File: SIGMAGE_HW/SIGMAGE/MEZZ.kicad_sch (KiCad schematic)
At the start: 4 parts, among them J12 61306421821, J13 61306421121, J14 61306421821, J8 61306421121

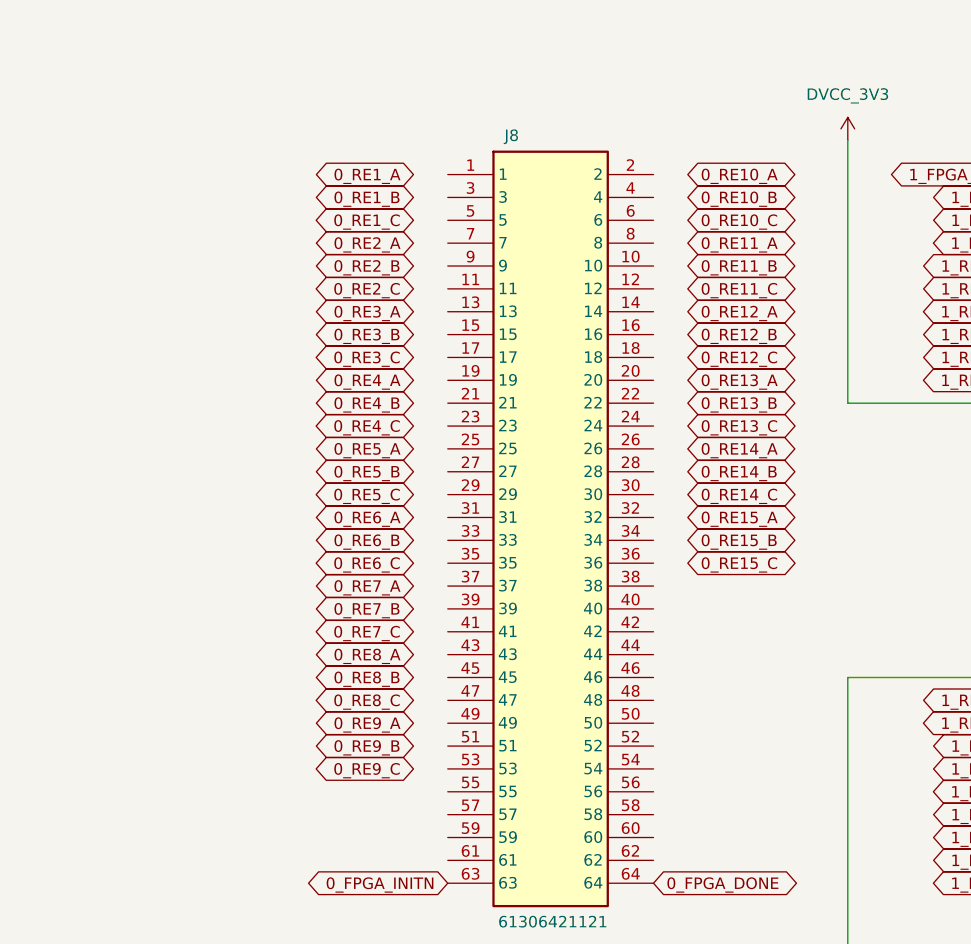
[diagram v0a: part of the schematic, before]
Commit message: foo bar
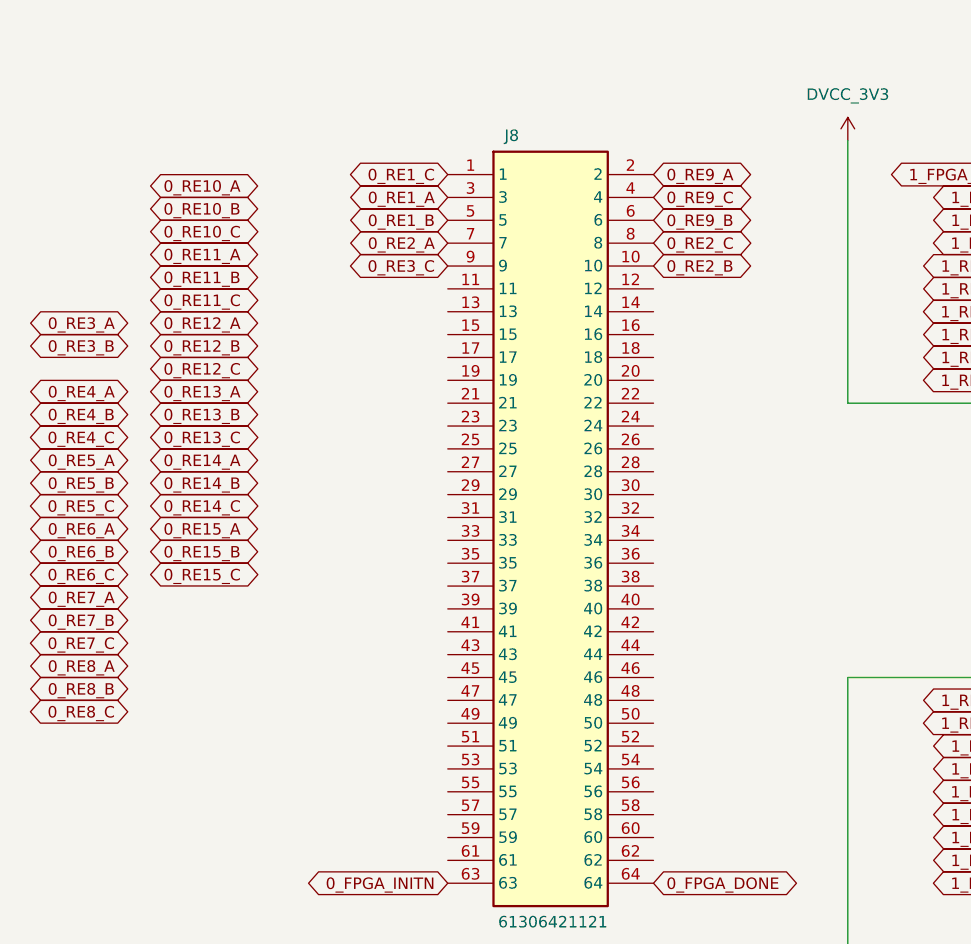
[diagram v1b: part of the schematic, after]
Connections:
- net 0_RE1_A: now also J8.3
- net 0_RE1_B: now also J8.5
- net 0_RE1_C: now also J8.1
- net 0_RE2_A: now also J8.7
- net 0_RE2_B: now also J8.10
- net 0_RE2_C: now also J8.8
- net 0_RE3_C: now also J8.9
- net 0_RE9_A: now also J8.2
- net 0_RE9_B: now also J8.6
- net 0_RE9_C: now also J8.4

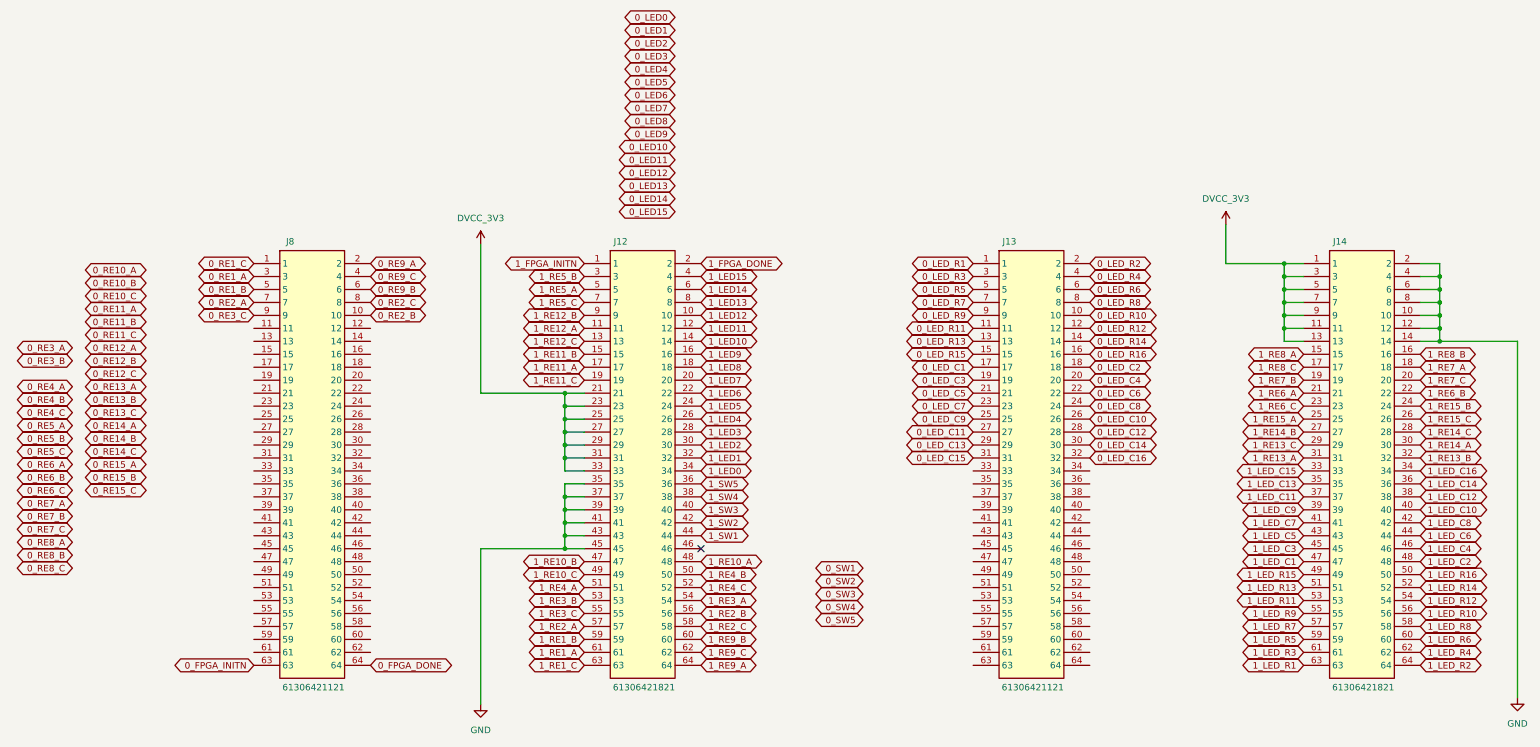
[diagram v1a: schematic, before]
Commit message: more routing
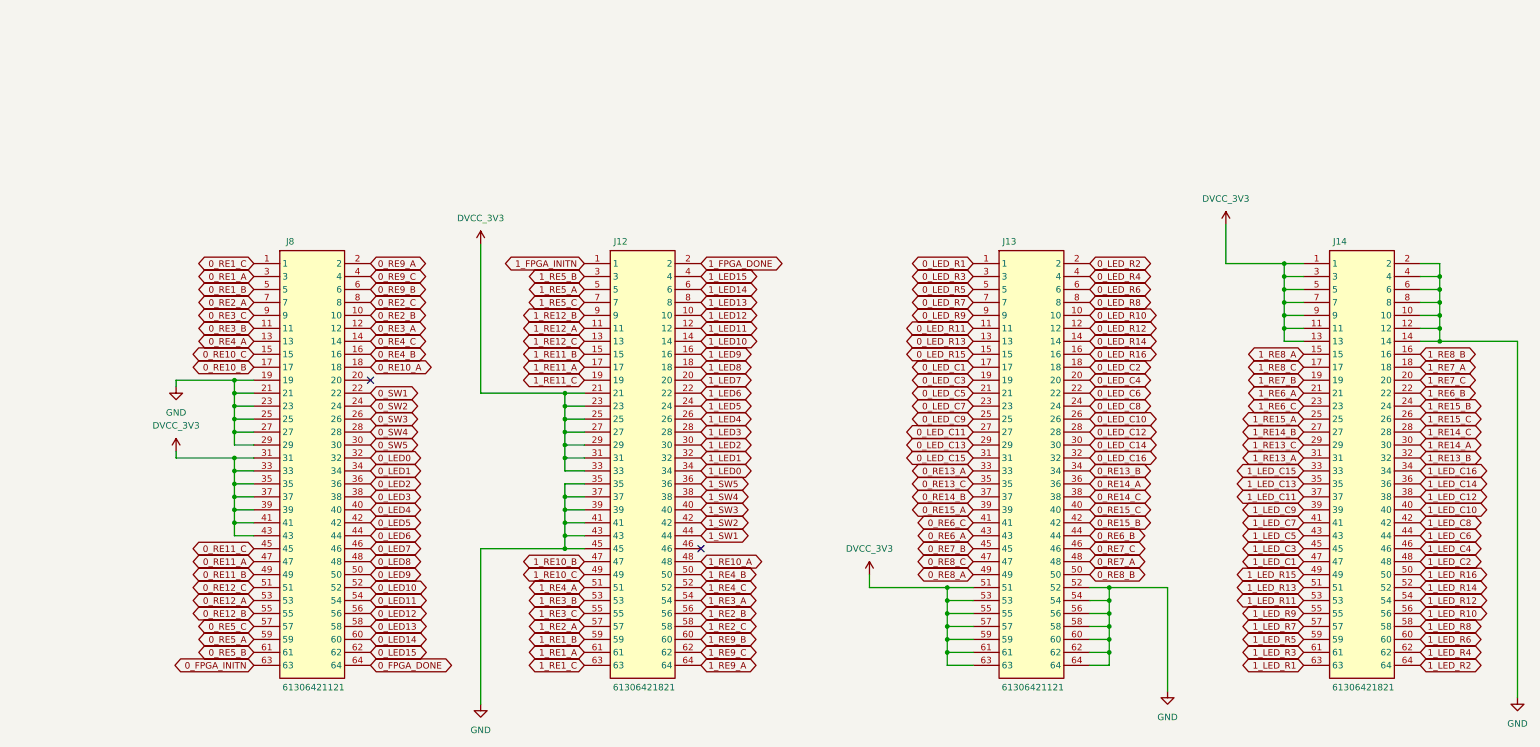
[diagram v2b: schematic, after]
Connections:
- net 0_LED0: now also J8.32
- net 0_LED1: now also J8.34
- net 0_LED10: now also J8.52
- net 0_LED11: now also J8.54
- net 0_LED12: now also J8.56
- net 0_LED13: now also J8.58
- net 0_LED14: now also J8.60
- net 0_LED15: now also J8.62
- net 0_LED2: now also J8.36
- net 0_LED3: now also J8.38
- net 0_LED4: now also J8.40
- net 0_LED5: now also J8.42
- net 0_LED6: now also J8.44
- net 0_LED7: now also J8.46
- net 0_LED8: now also J8.48
- net 0_LED9: now also J8.50
- net 0_RE10_A: now also J8.18
- net 0_RE10_B: now also J8.17
- net 0_RE10_C: now also J8.15
- net 0_RE11_A: now also J8.47
- net 0_RE11_B: now also J8.49
- net 0_RE11_C: now also J8.45
- net 0_RE12_A: now also J8.53
- net 0_RE12_B: now also J8.55
- net 0_RE12_C: now also J8.51
- net 0_RE13_A: now also J13.33
- net 0_RE13_B: now also J13.34
- net 0_RE13_C: now also J13.35
- net 0_RE14_A: now also J13.36
- net 0_RE14_B: now also J13.37
- net 0_RE14_C: now also J13.38
- net 0_RE15_A: now also J13.39
- net 0_RE15_B: now also J13.42
- net 0_RE15_C: now also J13.40
- net 0_RE3_A: now also J8.12
- net 0_RE3_B: now also J8.11
- net 0_RE4_A: now also J8.13
- net 0_RE4_B: now also J8.16
- net 0_RE4_C: now also J8.14
- net 0_RE5_A: now also J8.59
- net 0_RE5_B: now also J8.61
- net 0_RE5_C: now also J8.57
- net 0_RE6_A: now also J13.43
- net 0_RE6_B: now also J13.44
- net 0_RE6_C: now also J13.41
- net 0_RE7_A: now also J13.48
- net 0_RE7_B: now also J13.45
- net 0_RE7_C: now also J13.46
- net 0_RE8_A: now also J13.49
- net 0_RE8_B: now also J13.50
- net 0_RE8_C: now also J13.47
- net 0_SW1: now also J8.22
- net 0_SW2: now also J8.24
- net 0_SW3: now also J8.26
- net 0_SW4: now also J8.28
- net 0_SW5: now also J8.30
- net DVCC_3V3: now also J13.51, J13.53, J13.55, J13.57, J13.59, J13.61, J13.63, J8.31, J8.33, J8.35, J8.37, J8.39, J8.41, J8.43
- net GND: now also J13.52, J13.54, J13.56, J13.58, J13.60, J13.62, J13.64, J8.19, J8.21, J8.23, J8.25, J8.27, J8.29
- no-connect marks 1 -> 2

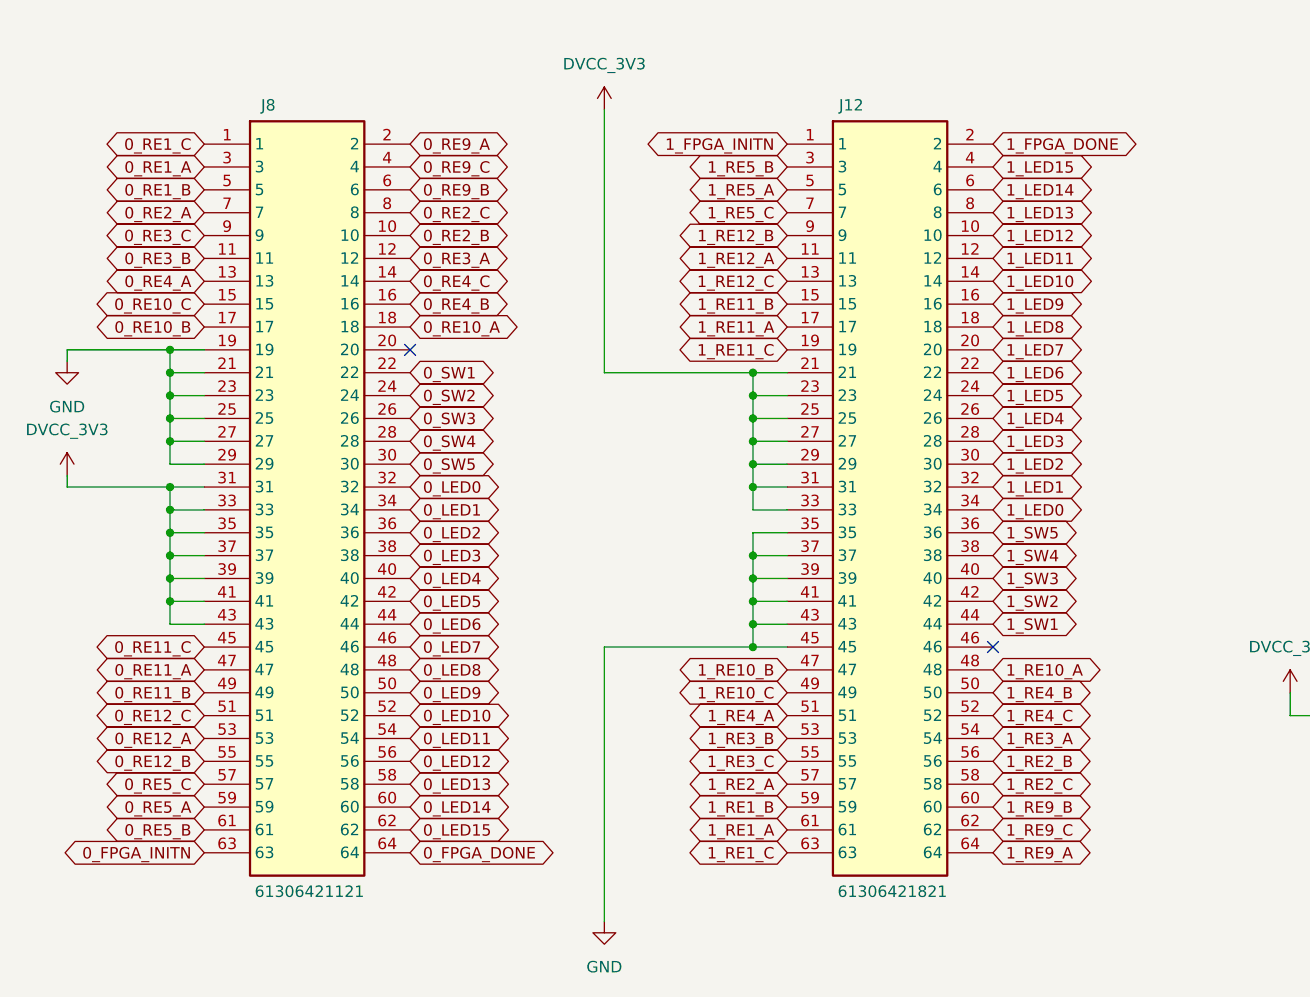
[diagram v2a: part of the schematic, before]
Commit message: some more power stuff
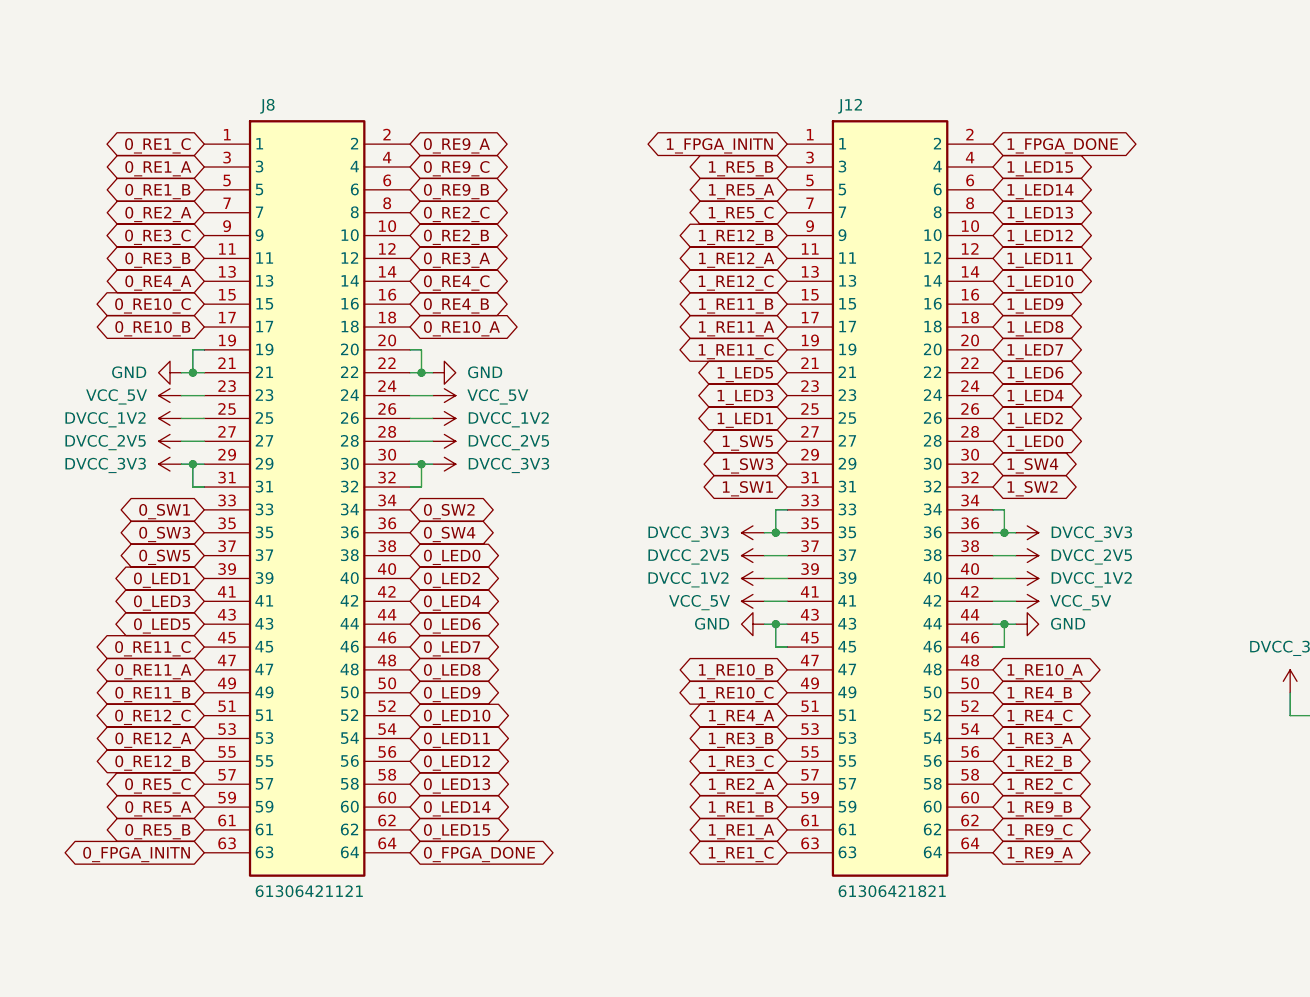
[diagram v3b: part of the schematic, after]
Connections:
- net 0_LED0: now also J8.38; no longer J8.32
- net 0_LED1: now also J8.39; no longer J8.34
- net 0_LED2: now also J8.40; no longer J8.36
- net 0_LED3: now also J8.41; no longer J8.38
- net 0_LED4: now also J8.42; no longer J8.40
- net 0_LED5: now also J8.43; no longer J8.42
- net 0_SW1: now also J8.33; no longer J8.22
- net 0_SW2: now also J8.34; no longer J8.24
- net 0_SW3: now also J8.35; no longer J8.26
- net 0_SW4: now also J8.36; no longer J8.28
- net 0_SW5: now also J8.37; no longer J8.30
- net 1_LED0: now also J12.28; no longer J12.34
- net 1_LED1: now also J12.25; no longer J12.32
- net 1_LED2: now also J12.26; no longer J12.30
- net 1_LED3: now also J12.23; no longer J12.28
- net 1_LED4: now also J12.24; no longer J12.26
- net 1_LED5: now also J12.21; no longer J12.24
- net 1_SW1: now also J12.31; no longer J12.44
- net 1_SW2: now also J12.32; no longer J12.42
- net 1_SW3: now also J12.29; no longer J12.40
- net 1_SW4: now also J12.30; no longer J12.38
- net 1_SW5: now also J12.27; no longer J12.36
- net DVCC_3V3: now also J12.34, J12.35, J12.36, J8.29, J8.30, J8.32; no longer J12.21, J12.23, J12.25, J12.27, J12.29, J12.31, J8.33, J8.35, J8.37, J8.39, J8.41, J8.43
- net GND: now also J12.44, J12.46, J8.20, J8.22; no longer J12.35, J12.37, J12.39, J12.41, J8.23, J8.25, J8.27, J8.29
- new net DVCC_1V2: J12.39, J12.40, J8.25, J8.26
- new net DVCC_2V5: J12.37, J12.38, J8.27, J8.28
- new net VCC_5V: J12.41, J12.42, J8.23, J8.24
- no-connect marks 2 -> 0
